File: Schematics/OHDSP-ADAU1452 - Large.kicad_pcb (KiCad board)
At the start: 2 copper layers, 100 x 100 mm, 305 parts, among them CN201 COAX, CN401 COAX, CN402 COAX, CN405 COAX, CN406 COAX, P201 CONN_2x1, P202 CONN_2x1, P203 CONN_6X2, P204 CONN_6x1, P301 CONN_2x1, P302 CONN_2x1, P303 PIN, P304 PIN, P305 PIN, P306 PIN, P601 CONN_02X05, P602 CONN_02X05, P603 CONN_02X05, P604 CONN_02X05, P605 CONN_3x1, P606 CONN_6X2, P607 CONN_02X05, P608 CONN_02X05, P609 CONN_02X20, P610 CONN_02X05, P611 CONN_5x1, P613 CONN_02X05, P614 CONN_02X05, P615 CONN_02X05, P616 CONN_02X05, SW201 SWITCH, SW202 SWITCH, U201 ADAU1452WBCPZ, U202 ADM13307-5ARZ, U203 25AA1024, U301 IC-REG-XRP7659ISTR-F, U302 IC-REG-XRP7659ISTR-F, U304 IC-REG-XC6210B332MR, U305 IC-REG-XC6210B332MR, U401 NB3L553, U501 IC-SPDIF-RX-OPTO, U502 IC-SPDIF-TX-OPTO, X201 24M576

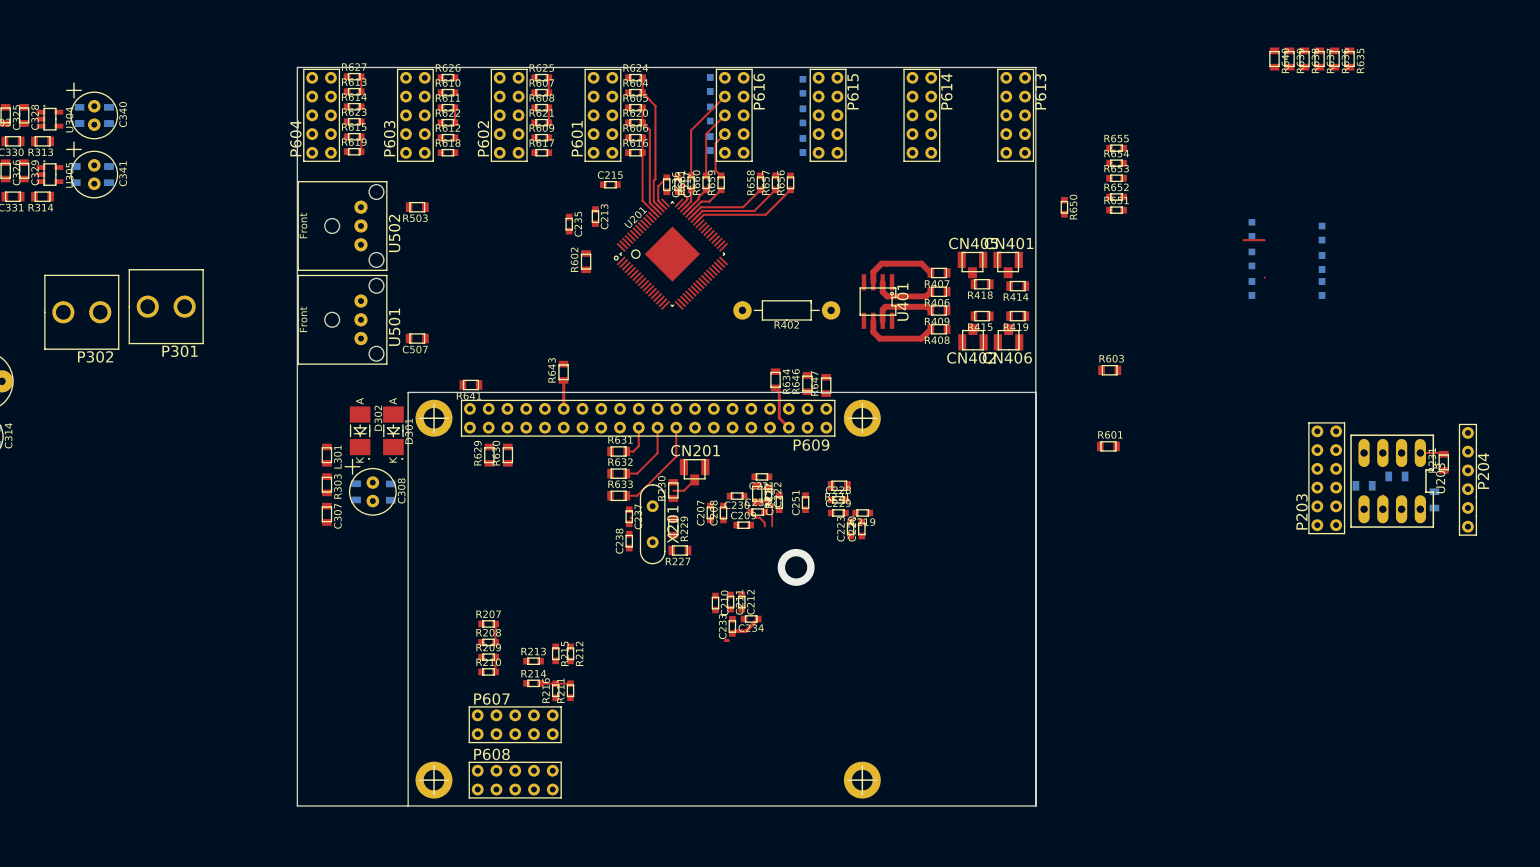
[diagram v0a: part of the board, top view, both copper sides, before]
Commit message: Revert "Going 4 layer on smaller PCB"
This reverts commit d1ec277a0becb058c7967dba94e28e7f31b1a00f.
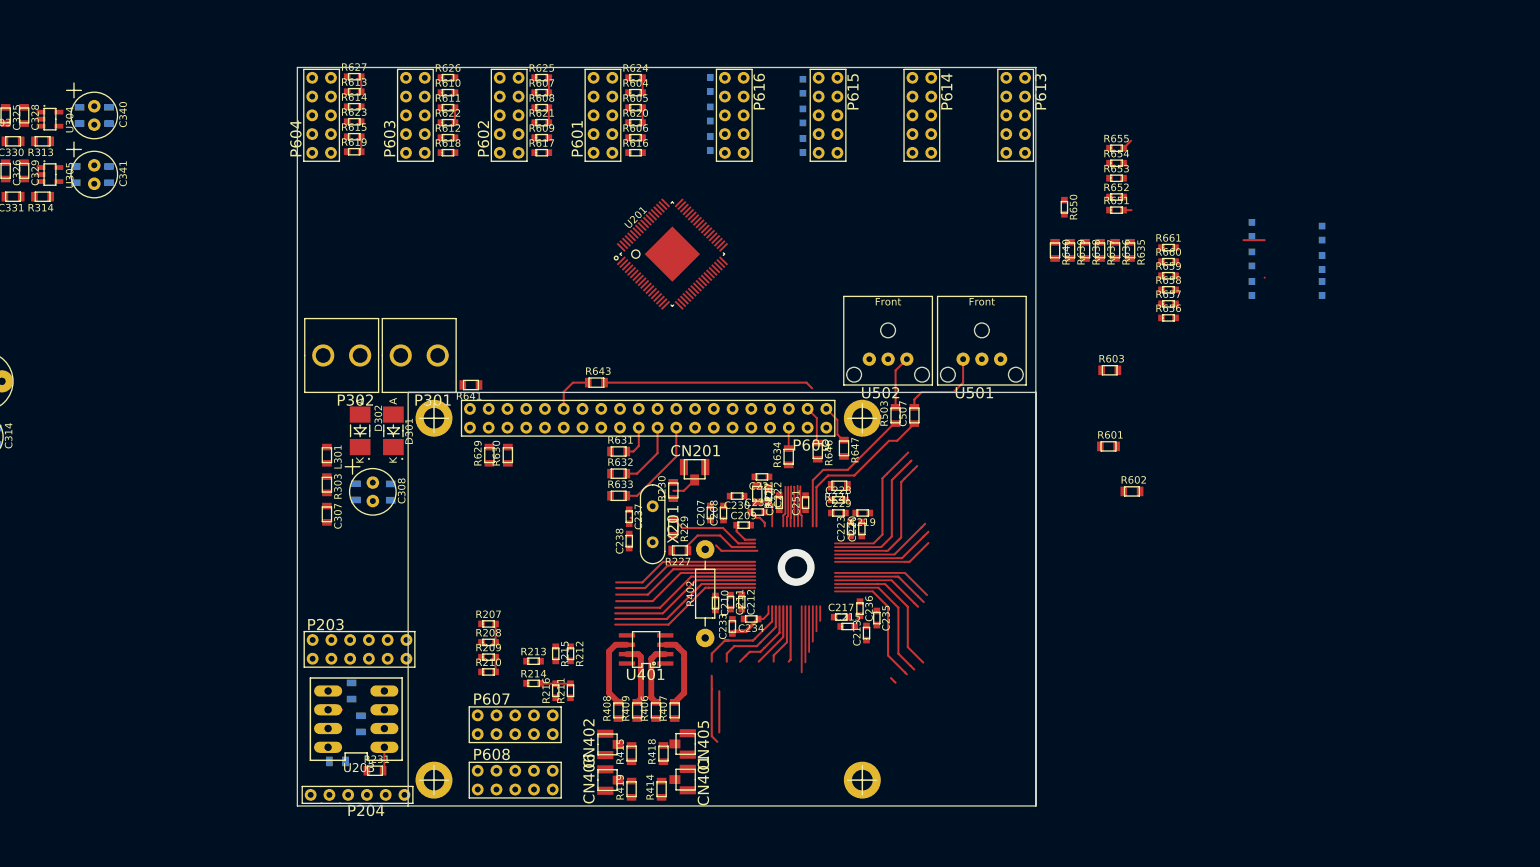
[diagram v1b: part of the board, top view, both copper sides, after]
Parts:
- moved C252 152.7 mm to (210.4, 118.0), turned to 0 degrees
- moved P204 152.1 mm to (219.5, 122.5), turned to 180 degrees
- moved R231 150.6 mm to (215.5, 119.2), turned to 0 degrees
- moved R232 144.2 mm to (213.6, 112.9), turned to 90 degrees
- moved U203 143.9 mm to (213.0, 112.2), turned to 180 degrees
- moved C254 139.9 mm to (212.3, 108.4), turned to 90 degrees
- moved P203 133.0 mm to (213.4, 102.8), turned to 270 degrees
- moved U501 84.2 mm to (297.7, 63.5), turned to 90 degrees
- moved R414 83.5 mm to (254.3, 121.7), turned to 90 degrees
- moved CN406 83.4 mm to (246.7, 122.5), turned to 90 degrees
- moved R419 82.7 mm to (250.3, 121.7), turned to 90 degrees
- moved R602 80.2 mm to (318.0, 81.4), turned to 0 degrees
- moved CN401 79.9 mm to (257.9, 118.4), turned to 270 degrees
- moved R418 76.8 mm to (254.6, 116.9), turned to 90 degrees
- moved CN402 76.6 mm to (246.7, 117.7), turned to 90 degrees
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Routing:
- net (no net): track 27.4 -> 537.1 mm
- net /Connectors/RPI_BCLK: track 0.00 -> 28.4 mm
- net /ADAU1452/ADAU_SPDIF_RX: track 0.00 -> 22.1 mm
- net /ADAU1452/ADAU_SPDIF_TX: track 0.00 -> 20.8 mm
- net /ADAU1452/ADCIN_LRCLK0: track 18.8 -> 1.97 mm
- net /ADAU1452/DACOUT_LRCLK2: track 14.4 -> 0.06 mm
- net /ADAU1452/ADCIN_BCLK0: track 14.7 -> 1.97 mm
- net Net-(P616-Pad8): track 12.6 -> 0.06 mm
- net /ADAU1452/DACOUT_BCLK2: track 12.5 -> 0.00 mm
- net /ADAU1452/XTALIN: track 0.00 -> 12.5 mm
- net Net-(C507-Pad2): track 0.00 -> 11.8 mm
- net /ADAU1452/XTALOUT: track 0.00 -> 11.0 mm
- net /ADAU1452/ADCIN_SDATA0: track 11.0 -> 0.00 mm
- net /ADAU1452/DACOUT_SDATA2: track 10.7 -> 0.00 mm
- net Net-(P616-Pad6): track 9.25 -> 0.00 mm
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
